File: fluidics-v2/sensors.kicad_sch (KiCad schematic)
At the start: 21 parts, among them IC3 HSCDRRN001BDSA3, IC4 HSCDRRN001BDSA3, IC5 HSCDRRN001BDSA3, IC6 HSCDRRN001BDSA3, U10 LTC4316CMS-TRPBF

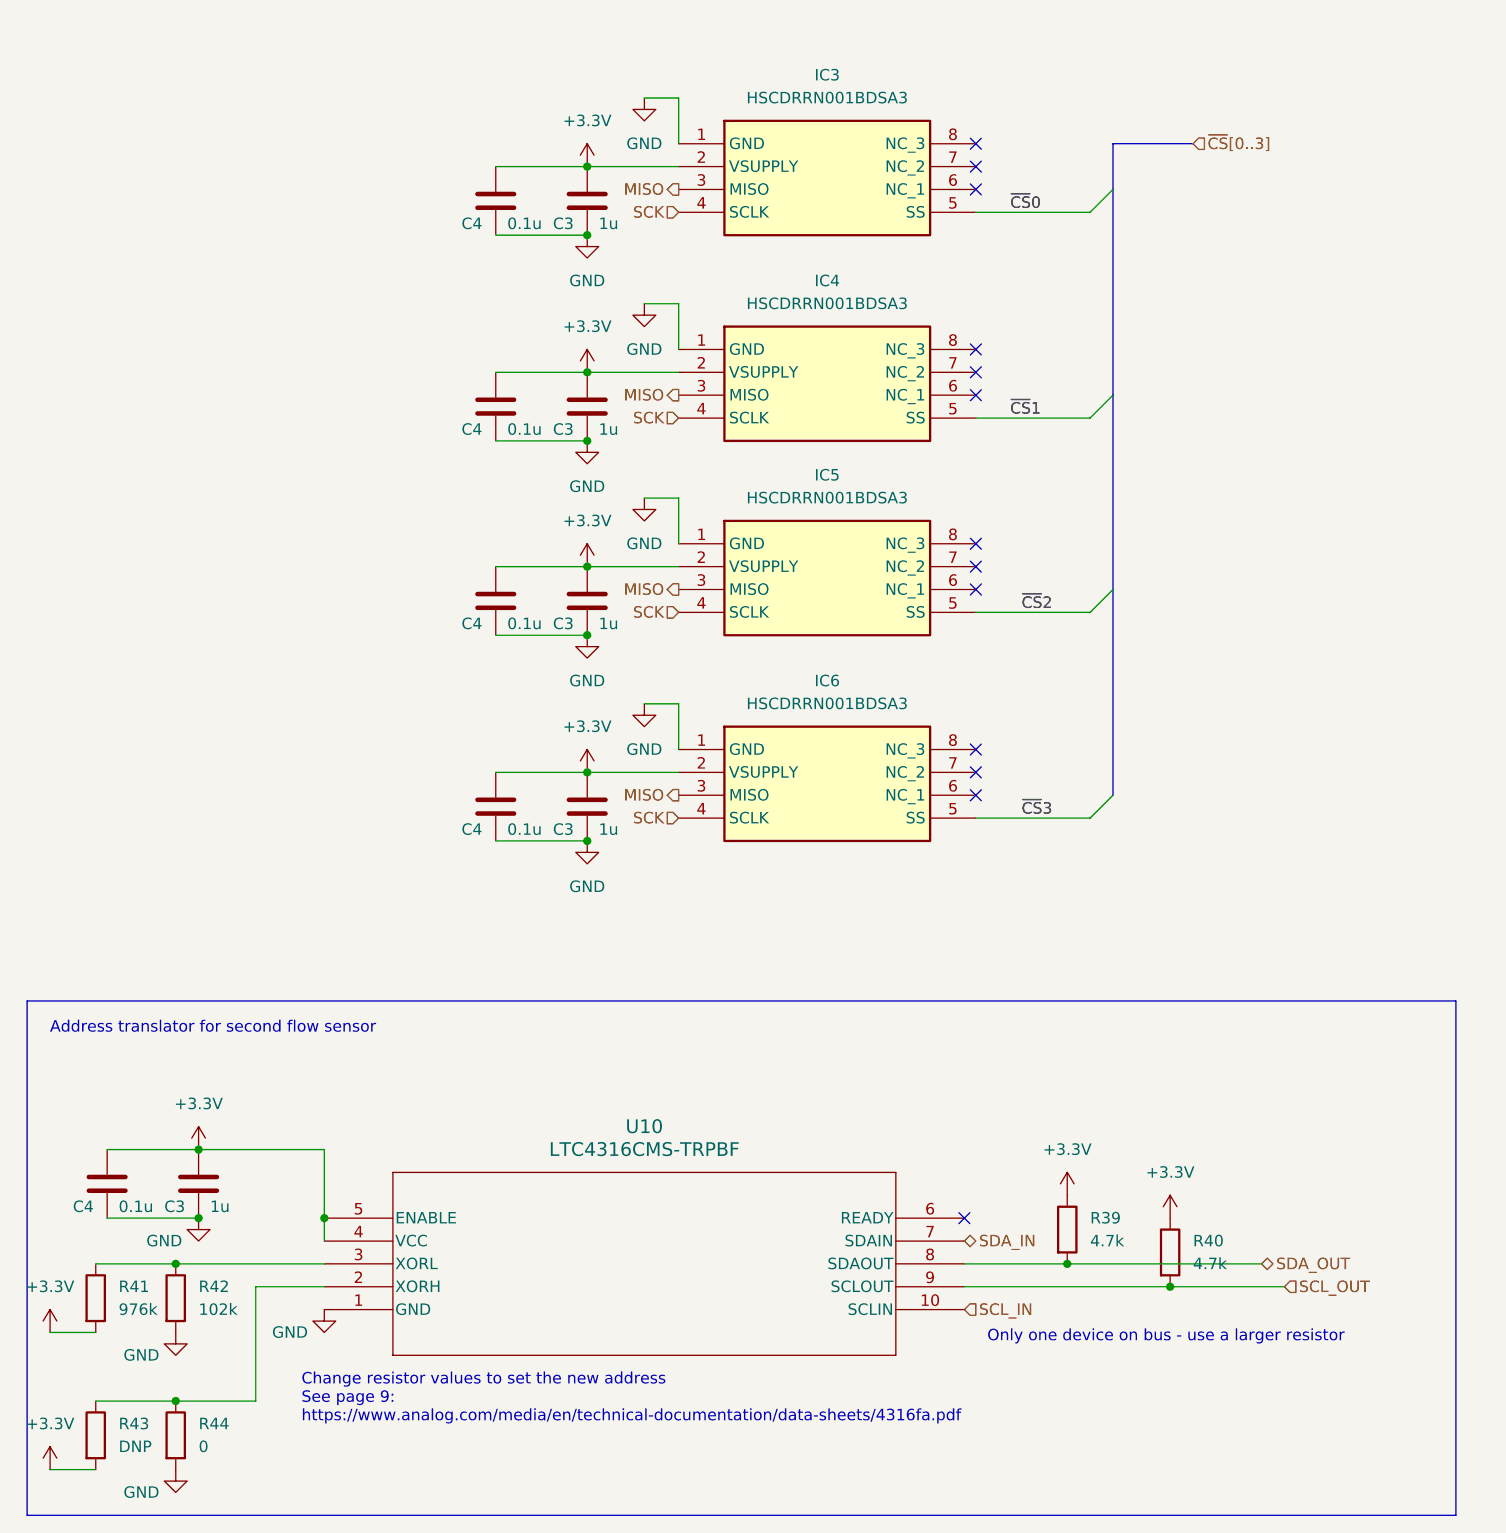
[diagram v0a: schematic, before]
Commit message: started layout
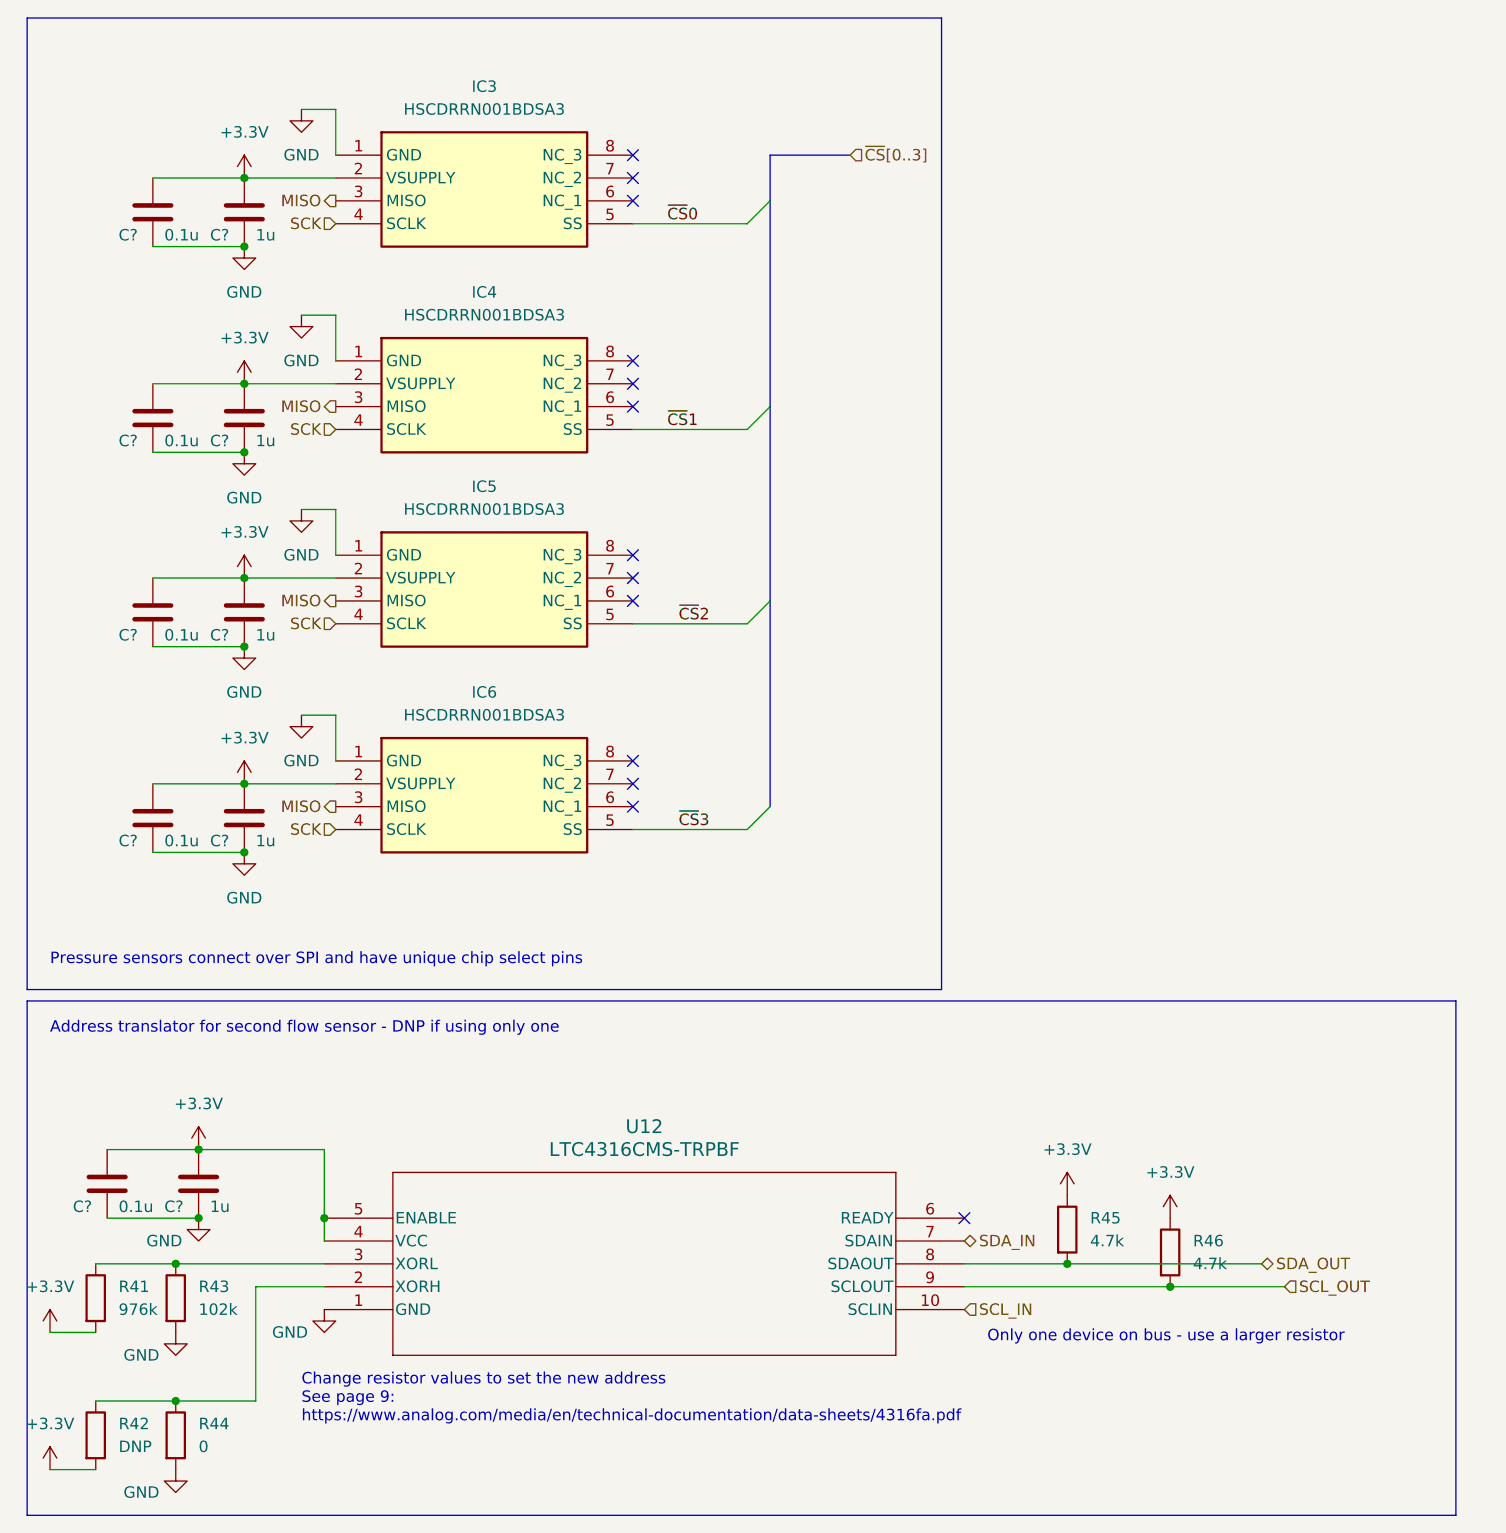
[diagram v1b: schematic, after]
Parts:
- IC3, IC4, IC5, IC6: footprint HSCDRRN001BDSA3 -> HSCDRRN001BDSA3:HSCDRRN001BDSA3
- renumbered C4 to C?, C3 to C?, R43 to R42, R42 to R43, R39 to R45, R40 to R46, U10 to U12
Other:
- note added: "Address translator for second flow sensor - DNP if using only one"
- note added: "Pressure sensors connect over SPI and have unique chip select pins"
- note removed: "Address translator for second flow sensor"
- moved on the sheet: C?, IC3
